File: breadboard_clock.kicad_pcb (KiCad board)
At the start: 2 copper layers, 106.7 x 35.6 mm, 27 parts, among them J101 Conn_01x02_Male, SW101 SW_Push, SW102 SW_SPDT, U101 ICM7555, U102 74LS04, U103 74LS04, U104 74LS08, U105 74LS32, U106 ICM7555, U107 74LS04, U108 ICM7555

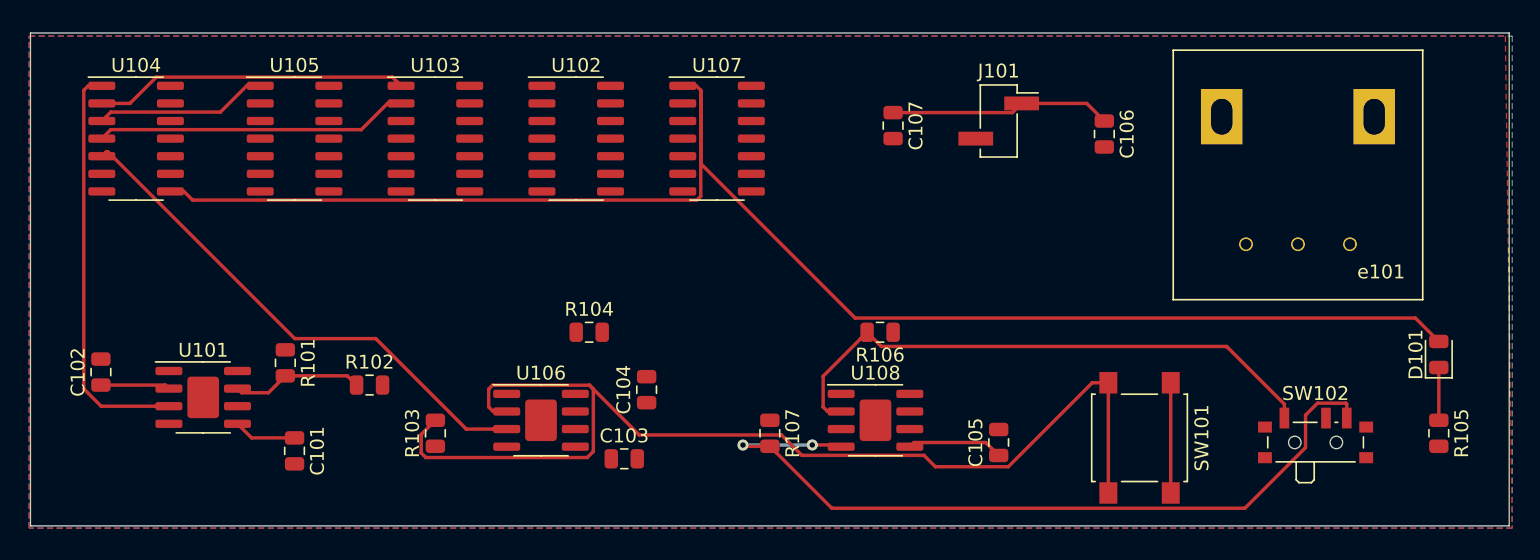
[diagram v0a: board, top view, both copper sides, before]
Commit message: Add files via upload
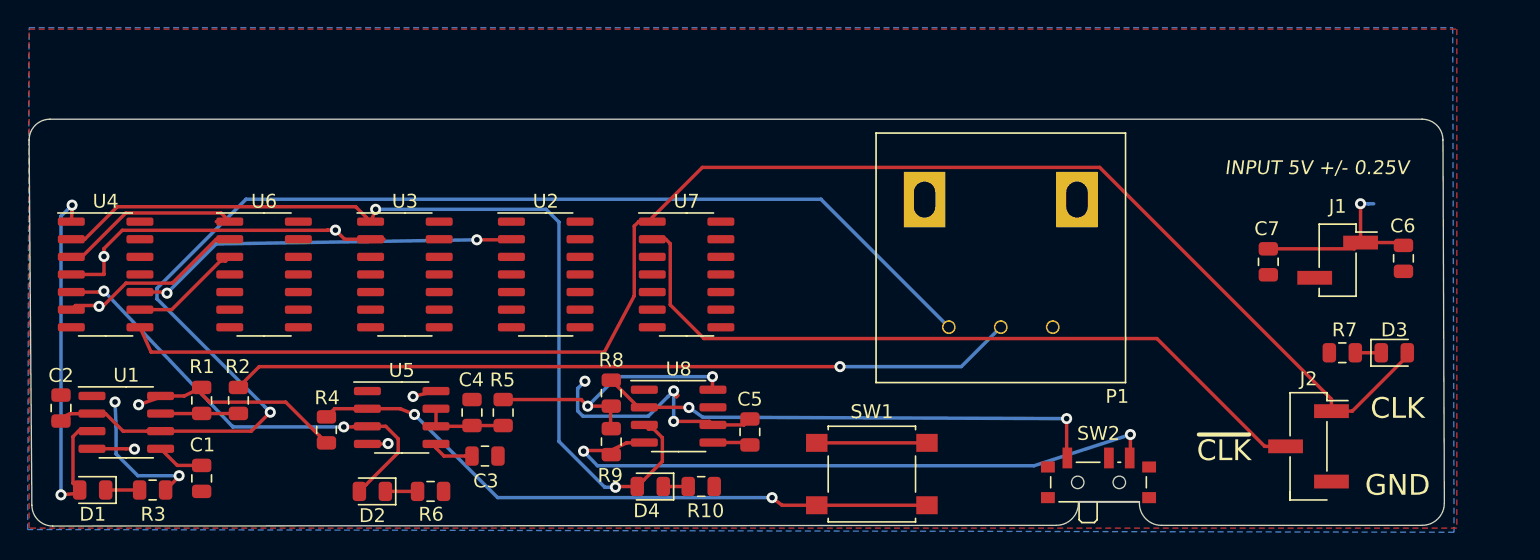
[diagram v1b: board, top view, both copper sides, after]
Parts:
- removed C106, C107: 0.1uF, Capacitor_SMD:C_0805_2012Metric
- removed J101: Conn_01x02_Male, Connector_PinHeader_2.54mm:PinHeader_1x02_P2.54mm_Vertical_SMD_Pin1Right
- removed R102: 1K, Resistor_SMD:R_0805_2012Metric
- removed U106: ICM7555, Package_SO:SOIC-8-1EP_3.9x4.9mm_P1.27mm_EP2.29x3mm
- removed e101: R_POT, Gerig-Added:Potentiomter_Bourns_PDB12_THT
- added C6: 0.1uF, Capacitor_SMD:C_0805_2012Metric, F.Cu at (137.2, 97.5)
- added C7: 0.1uF, Capacitor_SMD:C_0805_2012Metric, F.Cu at (127.4, 97.8)
- added D1: LED, LED_SMD:LED_0805_2012Metric, F.Cu at (42.6, 114.2)
- added D2: LED, LED_SMD:LED_0805_2012Metric, F.Cu at (62.8, 114.3)
- added D4: LED, LED_SMD:LED_0805_2012Metric, F.Cu at (82.8, 114.0)
- added J1: Conn_01x02_Male, Connector_PinHeader_2.54mm:PinHeader_1x02_P2.54mm_Vertical_SMD_Pin1Right, F.Cu at (132.4, 97.7)
- added J2: Conn_01x03_Male, Connector_PinHeader_2.54mm:PinHeader_1x03_P2.54mm_Vertical_SMD_Pin1Right, F.Cu at (130.3, 111.1)
- added P1: R_POT, Gerig-Added:Potentiomter_Bourns_PDB12_THT, F.Cu at (108.1, 102.5)
- added R10: 220, Resistor_SMD:R_0805_2012Metric, F.Cu at (86.5, 114.0)
- added R2: 1K, Resistor_SMD:R_0805_2012Metric, F.Cu at (53.1, 107.8)
- added R3: 220, Resistor_SMD:R_0805_2012Metric, F.Cu at (46.9, 114.2)
- added R6: 220, Resistor_SMD:R_0805_2012Metric, F.Cu at (67.0, 114.3)
- added U5: ICM7555, Package_SO:SOIC-8_3.9x4.9mm_P1.27mm, F.Cu at (64.9, 109.0)
- U1: renamed from U101; footprint Package_SO:SOIC-8-1EP_3.9x4.9mm_P1.27mm_EP2.29x3mm -> Package_SO:SOIC-8_3.9x4.9mm_P1.27mm
- U8: renamed from U108; footprint Package_SO:SOIC-8-1EP_3.9x4.9mm_P1.27mm_EP2.29x3mm -> Package_SO:SOIC-8_3.9x4.9mm_P1.27mm
- moved R8 19.9 mm to (80.0, 107.3), turned to 90 degrees
- moved SW1 19.5 mm to (98.8, 113.1), turned to 0 degrees
- moved C5 18.0 mm to (90.0, 110.1)
- moved SW2 15.9 mm to (115.2, 113.4)
- moved U8 14.2 mm to (84.9, 108.9)
- moved C4 12.7 mm to (70.0, 108.7)
- moved R9 11.5 mm to (80.0, 110.8)
- moved C3 10.1 mm to (70.9, 111.8)
- moved U2 10.0 mm to (75.3, 98.7)
- moved U3 10.0 mm to (65.1, 98.7)
- moved U4 10.0 mm to (43.5, 98.7)
- moved U6 10.0 mm to (55.0, 98.7)
- moved U7 10.0 mm to (85.4, 98.7)
- moved R7 9.07 mm to (132.7, 104.3), turned to 180 degrees
- moved R5 8.49 mm to (72.2, 108.7), turned to 270 degrees
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- renumbered C101 to C1, C102 to C2, C103 to C3, C104 to C4, C105 to C5, D101 to D3, R101 to R1, R103 to R4, R104 to R5, R105 to R7, R106 to R8, R107 to R9, SW101 to SW1, SW102 to SW2, U102 to U2, U103 to U3, U104 to U4, U105 to U6, U107 to U7
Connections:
- U2 pad 14: VCC -> (no net)
- U2 pad 7: GND -> (no net)
- U3 pad 14: VCC -> (no net)
- U3 pad 7: GND -> (no net)
- U4 pad 14: VCC -> (no net)
- U4 pad 7: GND -> (no net)
- U6 pad 14: VCC -> (no net)
- U6 pad 7: GND -> (no net)
- U7 pad 7: VCC -> (no net)
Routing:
- net Net-(C2-Pad1): track 5.01 -> 92.8 mm, vias 0 -> 1
- net Net-(P1-Pad2): track 0.00 -> 56.8 mm, vias 0 -> 1
- net ~CLK: track 0.00 -> 54.5 mm
- net Net-(D4-Pad2): track 22.6 -> 66.4 mm, vias 0 -> 2
- net VCC: track 16.0 -> 56.4 mm, vias 0 -> 7
- net Net-(R4-Pad2): track 80.9 -> 47.3 mm, vias 0 -> 2
- net GND: track 7.95 -> 36.8 mm, vias 0 -> 5
- net Net-(U2-Pad2): track 0.00 -> 28.4 mm, vias 0 -> 2
- net Net-(U4-Pad6): track 0.00 -> 13.5 mm, vias 0 -> 1
- net Net-(R9-Pad2): track 58.1 -> 46.7 mm
- net Net-(U4-Pad9): track 0.00 -> 8.06 mm
- net Net-(C4-Pad1): track 0.00 -> 6.14 mm
- net Net-(R8-Pad2): track 41.4 -> 36.7 mm, vias 0 -> 2
- net Net-(C5-Pad1): track 6.93 -> 2.74 mm
- net Net-(R1-Pad2): track 9.50 -> 5.62 mm
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- added copper zone on F.Cu, net GND
- added copper zone on B.Cu, net VCC
- removed copper zone on B.Cu, net GND
- removed copper zone on F.Cu, net VCC
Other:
- board size 106.7 x 35.6 mm -> 102.1 x 29.3 mm
- board text added: "CLK"
- board text added: "GND"
- board text added: "INPUT 5V +/- 0.25V"
- board text added: "~CLK"
